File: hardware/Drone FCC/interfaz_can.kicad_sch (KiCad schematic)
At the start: 22 parts, among them J801 CAN 1 Connector, J802 CAN 1 Connector, J803 CAN 2 Connector, J804 CAN 2 Connector, U801 SN65HVD230, U802 SN65HVD230

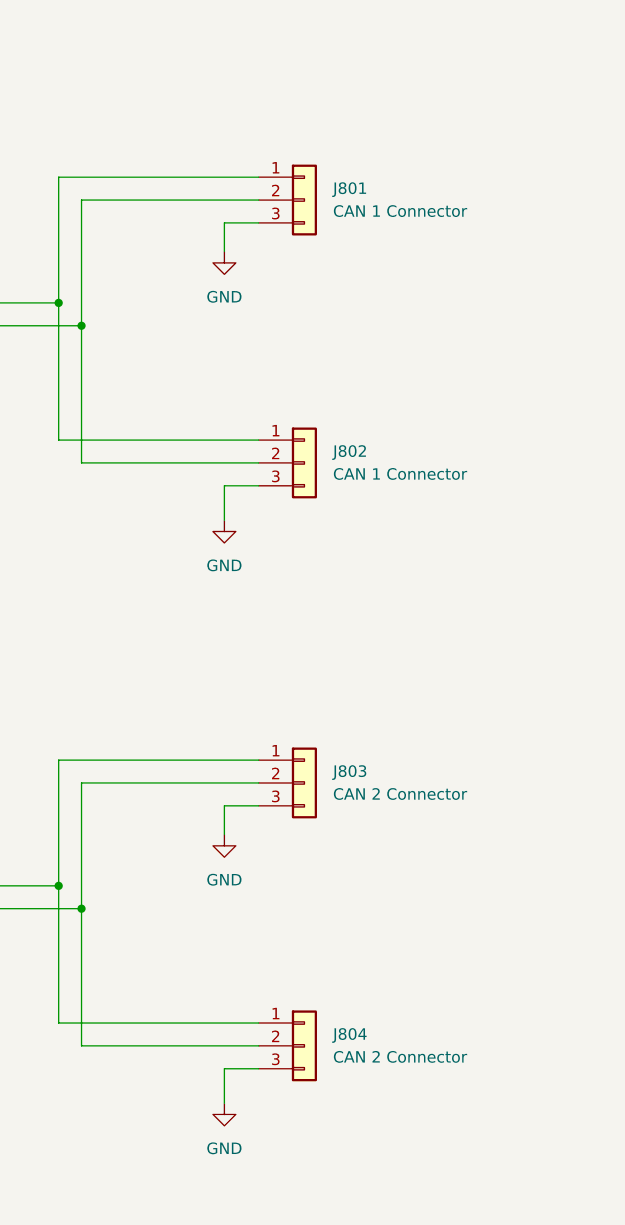
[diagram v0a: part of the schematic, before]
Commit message: start routing
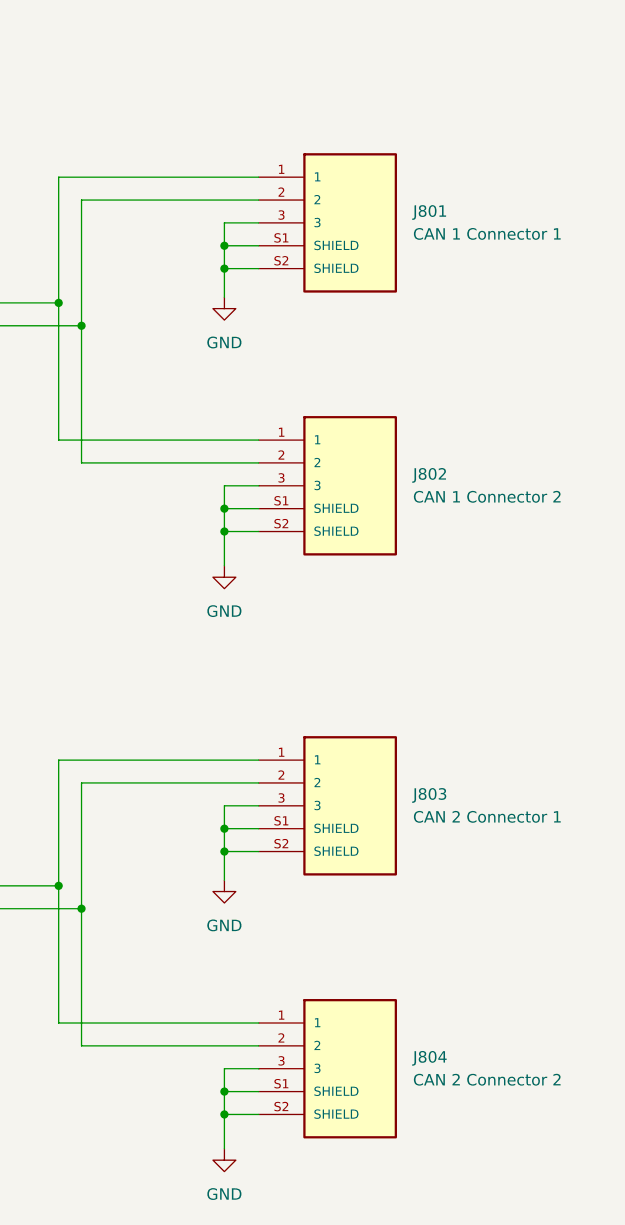
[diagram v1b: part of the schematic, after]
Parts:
- removed J801, J802: CAN 1 Connector, DF13A-3P-1.25H(21):HRS_DF13A-3P-1.25H(21), symbol Connector_Generic:Conn_01x03
- removed J803, J804: CAN 2 Connector, DF13A-3P-1.25H(21):HRS_DF13A-3P-1.25H(21), symbol Connector_Generic:Conn_01x03
- added J801: CAN 1 Connector 1, DF13A-3P-1.25H(21):HRS_DF13A-3P-1.25H(21), symbol DF13A-3P-1.25H(21):HRS_DF13A-3P-1.25H(21)
- added J802: CAN 1 Connector 2, DF13A-3P-1.25H(21):HRS_DF13A-3P-1.25H(21), symbol DF13A-3P-1.25H(21):HRS_DF13A-3P-1.25H(21)
- added J803: CAN 2 Connector 1, DF13A-3P-1.25H(21):HRS_DF13A-3P-1.25H(21), symbol DF13A-3P-1.25H(21):HRS_DF13A-3P-1.25H(21)
- added J804: CAN 2 Connector 2, DF13A-3P-1.25H(21):HRS_DF13A-3P-1.25H(21), symbol DF13A-3P-1.25H(21):HRS_DF13A-3P-1.25H(21)
- C801, C802, C804, C805: footprint (none) -> Capacitor_SMD:C_0603_1608Metric_Pad1.08x0.95mm_HandSolder
- C803, C806: footprint (none) -> Capacitor_SMD:C_0402_1005Metric_Pad0.74x0.62mm_HandSolder
- R801, R802, R803, R804, R805, R806, R807, R808: footprint (none) -> Resistor_SMD:R_0402_1005Metric_Pad0.72x0.64mm_HandSolder
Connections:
- net GND: now also J801.3, J801.S1 (SHIELD), J801.S2 (SHIELD), J802.3, J802.S1 (SHIELD), J802.S2 (SHIELD), J803.3, J803.S1 (SHIELD), J803.S2 (SHIELD), J804.3, J804.S1 (SHIELD), J804.S2 (SHIELD)
- net at D801.2 (A2), U801.6 (CANL): now also J801.2, J802.2
- net at D801.1 (A1), U801.7 (CANH): now also J801.1, J802.1
- net at D802.2 (A2), U802.6 (CANL): now also J803.2, J804.2
- net at D802.1 (A1), U802.7 (CANH): now also J803.1, J804.1
